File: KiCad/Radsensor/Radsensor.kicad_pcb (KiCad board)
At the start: 2 copper layers, 5 parts, among them Q1 Q_NPN_BCE

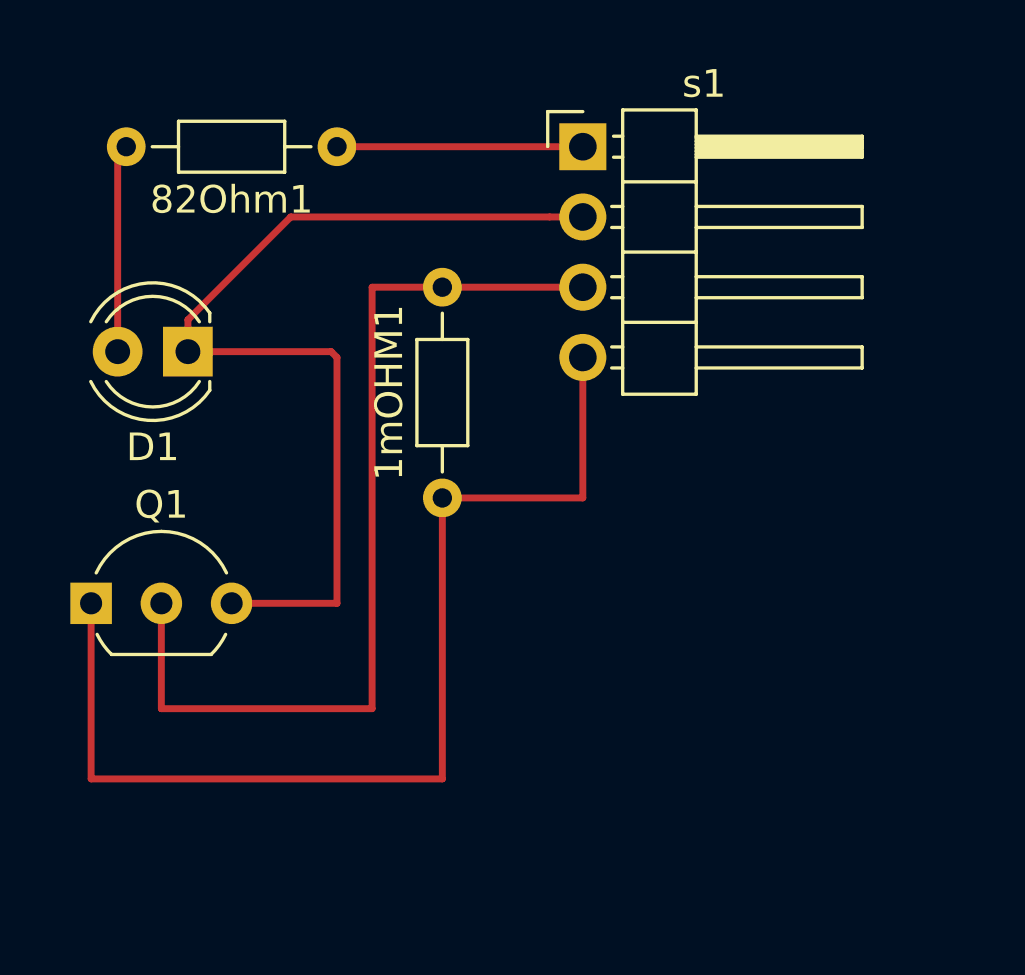
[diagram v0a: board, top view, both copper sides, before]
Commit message: Update der Platine
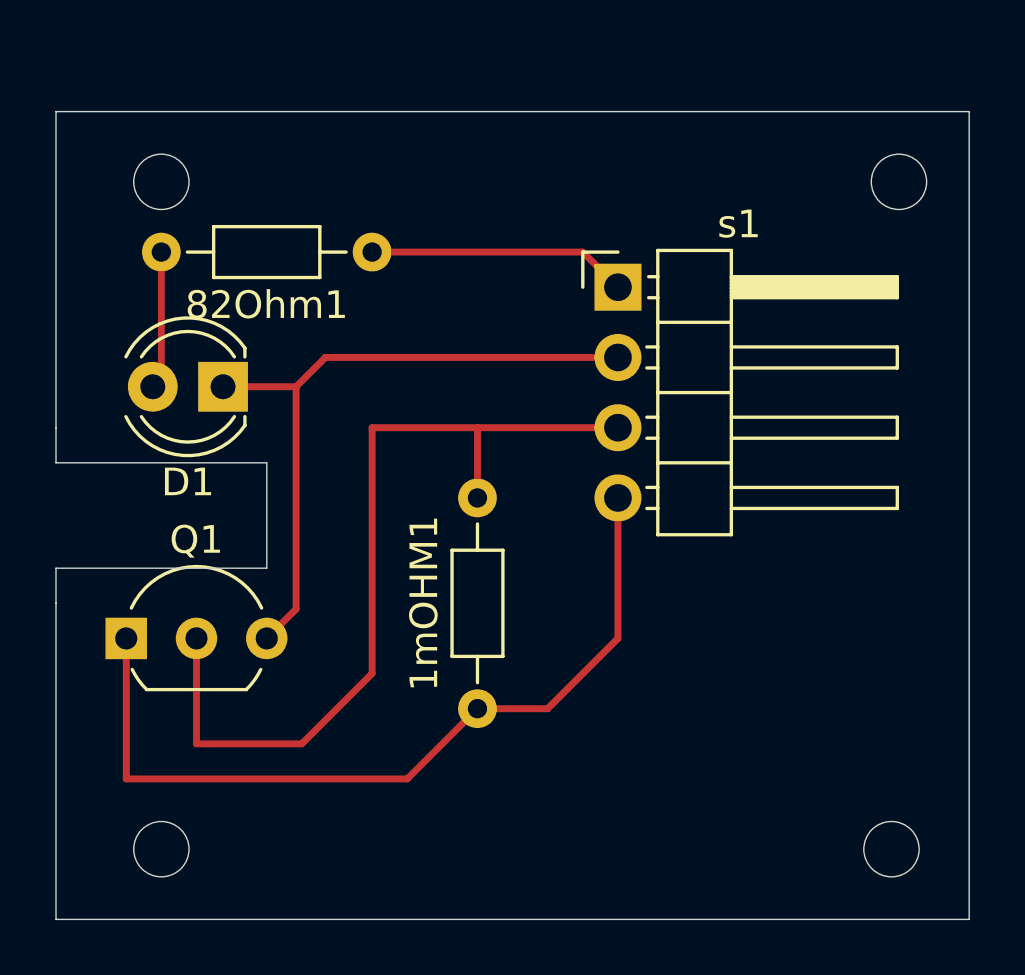
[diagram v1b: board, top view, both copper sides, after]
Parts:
- moved 1mOHM1 7.73 mm to (143.5, 43.2)
- moved s1 5.24 mm to (148.6, 27.9)
- moved 82Ohm1 4.02 mm to (139.7, 26.7)
- moved Q1 1.80 mm to (130.8, 40.6)
- moved D1 1.80 mm to (134.3, 31.5)
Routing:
- net Net-(D1-Pad1): track 35.1 -> 24.3 mm
- net Net-(1mOHM1-Pad1): track 39.4 -> 30.0 mm
- net Net-(1mOHM1-Pad2): track 34.3 -> 31.5 mm
- net Net-(82Ohm1-Pad2): track 7.54 -> 5.00 mm
- net Net-(82Ohm1-Pad1): track 8.89 -> 9.42 mm
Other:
- board outline added: 33 x 29.2 mm
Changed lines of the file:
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@@
   (general
     (thickness 1.6)
-    (drawings 0)
+    (drawings 14)
     (tracks 21)
     (zones 0)
@@
   )
   (module Resistor_THT:R_Axial_DIN0204_L3.6mm_D1.6mm_P7.62mm_Horizontal (layer F.Cu)
-    (at 142.24 35.56 90)
+    (at 143.51 43.18 90)
     (descr "Resistor, Axial_DIN0204 series, Axial, Horizontal, pin pitch=7.62mm, 0.167W, length*diameter=3.6*1.6mm^2, http://cdn-reichelt.de/documents/datenblatt/B400/1_4W%23YAG.pdf")
     (tags "Resistor Axial_DIN0204 series Axial Horizontal pin pitch 7.62mm 0.167W length 3.6mm diameter 1.6mm")
@@
   )
   (module Resistor_THT:R_Axial_DIN0204_L3.6mm_D1.6mm_P7.62mm_Horizontal (layer F.Cu)
-    (at 138.43 22.86 180)
+    (at 139.7 26.67 180)
     (descr "Resistor, Axial_DIN0204 series, Axial, Horizontal, pin pitch=7.62mm, 0.167W, length*diameter=3.6*1.6mm^2, http://cdn-reichelt.de/documents/datenblatt/B400/1_4W%23YAG.pdf")
     (tags "Resistor Axial_DIN0204 series Axial Horizontal pin pitch 7.62mm 0.167W length 3.6mm diameter 1.6mm")
@@
   )
   (module LED_THT:LED_D4.0mm (layer F.Cu)
-    (at 133.04 30.27 180)
+    (at 134.31 31.54 180)
     (descr "LED, diameter 4.0mm, 2 pins, http://www.kingbright.com/attachments/file/psearch/000/00/00/L-43GD(Ver.12B).pdf")
     (tags "LED diameter 4.0mm 2 pins")
@@
   )
   (module Package_TO_SOT_THT:TO-92_Inline_Wide (layer F.Cu)
-    (at 129.54 39.37)
+    (at 130.81 40.64)
     (descr "TO-92 leads in-line, wide, drill 0.75mm (see NXP sot054_po.pdf)")
     (tags "to-92 sc-43 sc-43a sot54 PA33 transistor")
@@
   )
   (module Connector_PinHeader_2.54mm:PinHeader_1x04_P2.54mm_Horizontal (layer F.Cu)
-    (at 147.32 22.86)
+    (at 148.59 27.94)
     (descr "Through hole angled pin header, 1x04, 2.54mm pitch, 6mm pin length, single row")
     (tags "Through hole angled pin header THT 1x04 2.54mm single row")
@@
     )
   )
-  (segment (start 142.24 45.72) (end 142.24 35.56) (width 0.25) (layer F.Cu) (net 1))
-  (segment (start 129.54 39.37) (end 129.54 45.72) (width 0.25) (layer F.Cu) (net 1))
-  (segment (start 129.54 45.72) (end 142.24 45.72) (width 0.25) (layer F.Cu) (net 1))
-  (segment (start 142.24 35.56) (end 147.32 35.56) (width 0.25) (layer F.Cu) (net 1))
-  (segment (start 147.32 35.56) (end 147.32 30.48) (width 0.25) (layer F.Cu) (net 1))
-  (segment (start 147.32 27.94) (end 142.24 27.94) (width 0.25) (layer F.Cu) (net 2))
-  (segment (start 142.24 27.94) (end 139.7 27.94) (width 0.25) (layer F.Cu) (net 2))
-  (segment (start 139.7 27.94) (end 139.7 43.18) (width 0.25) (layer F.Cu) (net 2))
-  (segment (start 139.7 43.18) (end 132.08 43.18) (width 0.25) (layer F.Cu) (net 2))
-  (segment (start 132.08 43.18) (end 132.08 39.37) (width 0.25) (layer F.Cu) (net 2))
-  (segment (start 130.5 23.17) (end 130.81 22.86) (width 0.25) (layer F.Cu) (net 3) (status 30))
-  (segment (start 130.5 30.27) (end 130.5 23.17) (width 0.25) (layer F.Cu) (net 3) (status 30))
-  (segment (start 147.32 22.86) (end 138.43 22.86) (width 0.25) (layer F.Cu) (net 4) (status 30))
-  (segment (start 146.117919 25.4) (end 147.32 25.4) (width 0.25) (layer F.Cu) (net 5) (status 20))
-  (segment (start 136.76 25.4) (end 146.117919 25.4) (width 0.25) (layer F.Cu) (net 5))
-  (segment (start 133.04 29.12) (end 136.76 25.4) (width 0.25) (layer F.Cu) (net 5))
-  (segment (start 133.04 30.27) (end 133.04 29.12) (width 0.25) (layer F.Cu) (net 5) (status 10))
-  (segment (start 138.43 39.37) (end 134.62 39.37) (width 0.25) (layer F.Cu) (net 5))
-  (segment (start 138.43 30.48) (end 138.43 39.37) (width 0.25) (layer F.Cu) (net 5))
-  (segment (start 133.04 30.27) (end 138.22 30.27) (width 0.25) (layer F.Cu) (net 5))
-  (segment (start 138.22 30.27) (end 138.43 30.48) (width 0.25) (layer F.Cu) (net 5))
+  (gr_line (start 135.89 38.1) (end 135.89 34.29) (layer Edge.Cuts) (width 0.05))
+  (gr_line (start 135.89 34.29) (end 128.27 34.29) (layer Edge.Cuts) (width 0.05))
+  (gr_line (start 128.27 38.1) (end 135.89 38.1) (layer Edge.Cuts) (width 0.05))
+  (gr_line (start 128.27 34.29) (end 128.27 33.02) (layer Edge.Cuts) (width 0.05))
+  (gr_line (start 128.27 39.37) (end 128.27 38.1) (layer Edge.Cuts) (width 0.05))
+  (gr_line (start 128.27 50.8) (end 128.27 39.37) (layer Edge.Cuts) (width 0.05))
+  (gr_line (start 128.27 21.59) (end 128.27 33.02) (layer Edge.Cuts) (width 0.05))
+  (gr_line (start 161.29 21.59) (end 128.27 21.59) (layer Edge.Cuts) (width 0.05))
+  (gr_line (start 161.29 50.8) (end 161.29 21.59) (layer Edge.Cuts) (width 0.05))
+  (gr_line (start 128.27 50.8) (end 161.29 50.8) (layer Edge.Cuts) (width 0.05))
+  (gr_circle (center 158.48 48.26) (end 159.48 48.26) (layer Edge.Cuts) (width 0.05))
+  (gr_circle (center 132.08 48.26) (end 133.08 48.26) (layer Edge.Cuts) (width 0.05))
+  (gr_circle (center 158.75 24.13) (end 159.75 24.13) (layer Edge.Cuts) (width 0.05))
+  (gr_circle (center 132.08 24.13) (end 133.08 24.13) (layer Edge.Cuts) (width 0.05))
+  (segment (start 140.97 45.72) (end 143.51 43.18) (width 0.25) (layer F.Cu) (net 1))
+  (segment (start 130.81 40.64) (end 130.81 45.72) (width 0.25) (layer F.Cu) (net 1))
+  (segment (start 130.81 45.72) (end 140.97 45.72) (width 0.25) (layer F.Cu) (net 1))
+  (segment (start 143.51 43.18) (end 146.05 43.18) (width 0.25) (layer F.Cu) (net 1))
+  (segment (start 148.59 40.64) (end 148.59 35.56) (width 0.25) (layer F.Cu) (net 1))
+  (segment (start 146.05 43.18) (end 148.59 40.64) (width 0.25) (layer F.Cu) (net 1))
+  (segment (start 139.7 33.02) (end 148.59 33.02) (width 0.25) (layer F.Cu) (net 2))
+  (segment (start 139.7 41.91) (end 139.7 33.02) (width 0.25) (layer F.Cu) (net 2))
+  (segment (start 137.16 44.45) (end 139.7 41.91) (width 0.25) (layer F.Cu) (net 2))
+  (segment (start 133.35 40.64) (end 133.35 44.45) (width 0.25) (layer F.Cu) (net 2))
+  (segment (start 133.35 44.45) (end 137.16 44.45) (width 0.25) (layer F.Cu) (net 2))
+  (segment (start 143.51 35.56) (end 143.51 33.02) (width 0.25) (layer F.Cu) (net 2))
+  (segment (start 132.08 31.23) (end 131.77 31.54) (width 0.25) (layer F.Cu) (net 3))
+  (segment (start 132.08 26.67) (end 132.08 31.23) (width 0.25) (layer F.Cu) (net 3))
+  (segment (start 148.59 27.94) (end 147.32 26.67) (width 0.25) (layer F.Cu) (net 4))
+  (segment (start 147.32 26.67) (end 139.7 26.67) (width 0.25) (layer F.Cu) (net 4))
+  (segment (start 136.95 39.58) (end 135.89 40.64) (width 0.25) (layer F.Cu) (net 5))
+  (segment (start 134.31 31.54) (end 136.95 31.54) (width 0.25) (layer F.Cu) (net 5))
+  (segment (start 136.95 31.54) (end 136.95 39.58) (width 0.25) (layer F.Cu) (net 5))
+  (segment (start 138.01 30.48) (end 136.95 31.54) (width 0.25) (layer F.Cu) (net 5))
+  (segment (start 148.59 30.48) (end 138.01 30.48) (width 0.25) (layer F.Cu) (net 5))
 )
